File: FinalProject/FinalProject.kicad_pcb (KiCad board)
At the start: 4 copper layers, 100 x 100 mm, 143 parts, among them J1 GSB4111312HR, J10 Conn_01x02, J2 GSB4111312HR, J3 GSB4111312HR, J5 ARJM11D7-502-AB-EW2, J6 DCJ200-10-A-XX-K_REVA, J7 Conn_01x02, J9 Conn_01x03, Q1 NTTFS5C673NLTAG, Q2 NTTFS5C673NLTAG, SW2 SW_Push, U1 RTL8153B-VB-CG, U11 RP2040, U12 TUSB8041, U14 NCP1117-3.3_SOT223, U15 VEML6040, U16 MAX98357A, U2 TPS2561DRCR, U3 LM74700, U4 TPS62902RPJR, U5 LM74700, U8 ABM8-272-T3, U9 W25Q128JVS, Y2 ABLS-25.000MHZ-B2F-T, Y3 ABM3C-24.000MHZ-D4Y-T

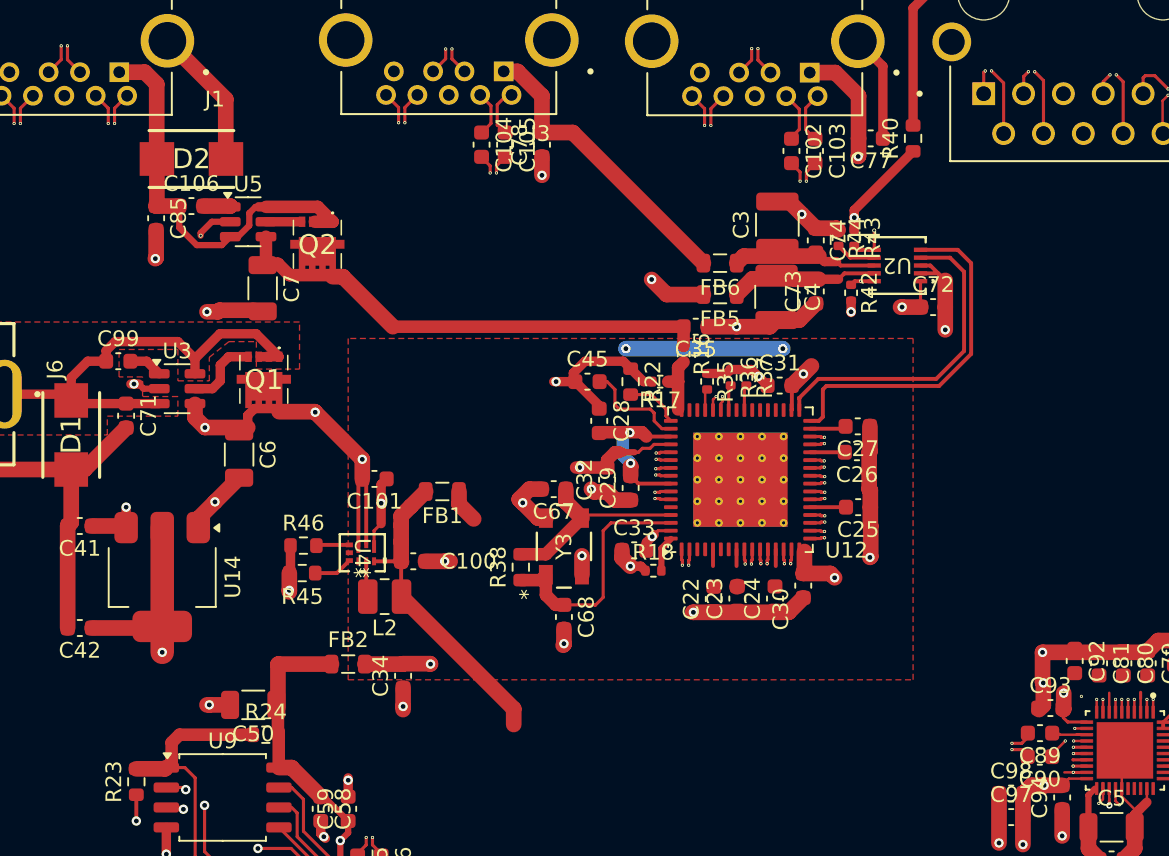
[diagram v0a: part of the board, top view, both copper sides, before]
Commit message: having DRC error
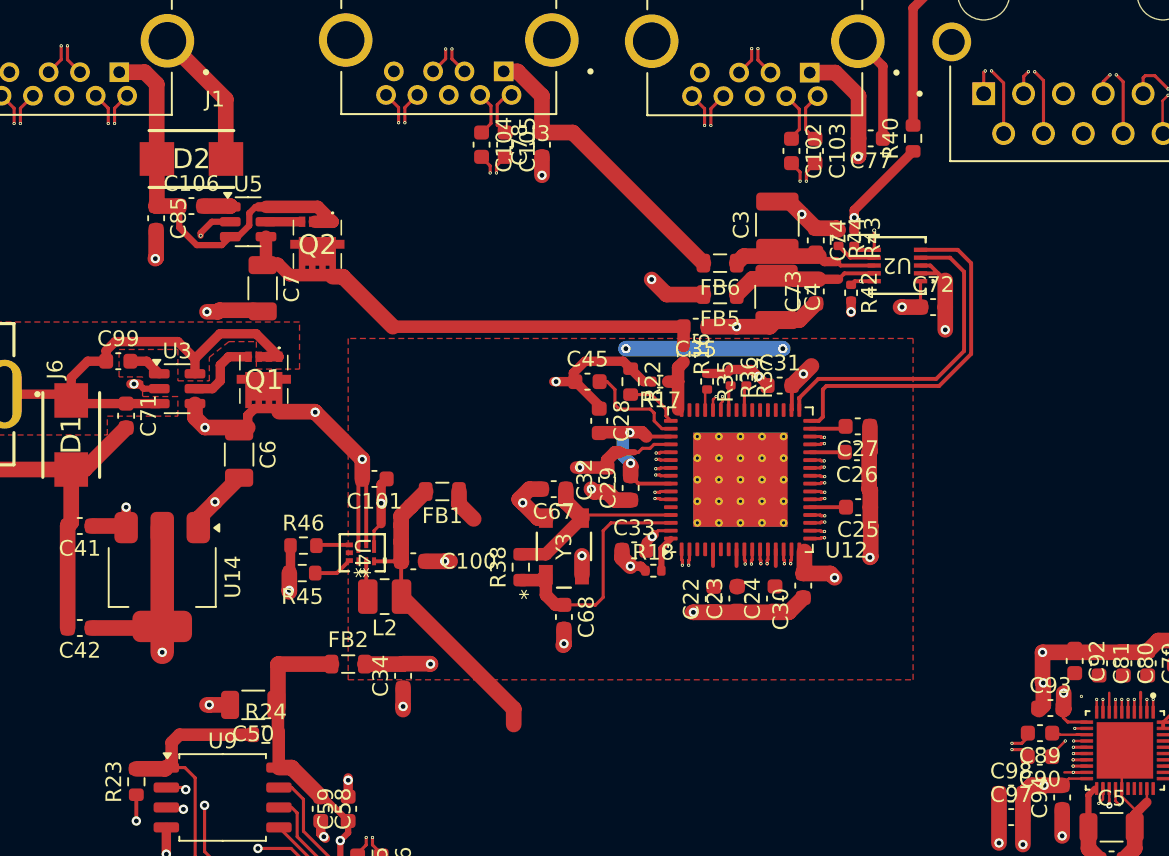
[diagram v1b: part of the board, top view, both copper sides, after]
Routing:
- net /DN1_D-: vias 1 -> 2
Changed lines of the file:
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@@
+	)
+	(via
+		(at 106.7 107.6)
+		(size 0.2)
+		(drill 0.1)
+		(layers "F.Cu" "B.Cu")
+		(net 101)
 	)
 	(via
@@
 	)
 	(segment
+		(start 81.0625 91)
+		(end 80.406249 91)
+		(width 0.2)
+		(layer "F.Cu")
+		(net 141)
+	)
+	(segment
 		(start 39.2125 67.05)
 		(end 39.2125 66.08)
@@
 		(start 39.2125 66.08)
 		(end 38.4125 65.28)
-		(width 0.2)
-		(layer "F.Cu")
-		(net 141)
-	)
-	(segment
-		(start 81.0625 91)
-		(end 80.406249 91)
 		(width 0.2)
 		(layer "F.Cu")
@@
 	)
 	(segment
+		(start 39.2125 68.245344)
+		(end 40.317156 69.35)
+		(width 0.2)
+		(layer "In2.Cu")
+		(net 141)
+	)
+	(segment
+		(start 68.517156 94)
+		(end 74.082844 94)
+		(width 0.2)
+		(layer "In2.Cu")
+		(net 141)
+	)
+	(segment
+		(start 77.132844 90.95)
+		(end 80.05 90.95)
+		(width 0.2)
+		(layer "In2.Cu")
+		(net 141)
+	)
+	(segment
+		(start 74.082844 94)
+		(end 77.132844 90.95)
+		(width 0.2)
+		(layer "In2.Cu")
+		(net 141)
+	)
+	(segment
+		(start 39.2125 67.05)
+		(end 39.2125 68.245344)
+		(width 0.2)
+		(layer "In2.Cu")
+		(net 141)
+	)
+	(segment
+		(start 43.867156 69.35)
+		(end 68.517156 94)
+		(width 0.2)
+		(layer "In2.Cu")
+		(net 141)
+	)
+	(segment
 		(start 40.317156 69.35)
-		(end 39.2125 68.245344)
-		(width 0.2)
-		(layer "In2.Cu")
-		(net 141)
-	)
-	(segment
-		(start 68.517156 94)
 		(end 43.867156 69.35)
-		(width 0.2)
-		(layer "In2.Cu")
-		(net 141)
-	)
-	(segment
-		(start 77.132844 90.95)
-		(end 74.082844 94)
-		(width 0.2)
-		(layer "In2.Cu")
-		(net 141)
-	)
-	(segment
-		(start 80.05 90.95)
-		(end 77.132844 90.95)
-		(width 0.2)
-		(layer "In2.Cu")
-		(net 141)
-	)
-	(segment
-		(start 74.082844 94)
-		(end 68.517156 94)
-		(width 0.2)
-		(layer "In2.Cu")
-		(net 141)
-	)
-	(segment
-		(start 39.2125 68.245344)
-		(end 39.2125 67.05)
-		(width 0.2)
-		(layer "In2.Cu")
-		(net 141)
-	)
-	(segment
-		(start 43.867156 69.35)
-		(end 40.317156 69.35)
 		(width 0.2)
 		(layer "In2.Cu")
@@
 	)
 	(segment
+		(start 45.2125 66.08)
+		(end 45.2125 67.05)
+		(width 0.2)
+		(layer "F.Cu")
+		(net 144)
+	)
+	(segment
 		(start 80.406249 89.5)
 		(end 80.356249 89.45)
@@
 	)
 	(segment
-		(start 45.2125 67.05)
+		(start 44.4125 65.28)
 		(end 45.2125 66.08)
-		(width 0.2)
-		(layer "F.Cu")
-		(net 144)
-	)
-	(segment
-		(start 45.2125 66.08)
-		(end 44.4125 65.28)
 		(width 0.2)
 		(layer "F.Cu")
@@
 	)
 	(segment
+		(start 79.182844 89.45)
+		(end 80.1 89.45)
+		(width 0.2)
+		(layer "In2.Cu")
+		(net 144)
+	)
+	(segment
+		(start 78.75413 89.878714)
+		(end 79.182844 89.45)
+		(width 0.2)
+		(layer "In2.Cu")
+		(net 144)
+	)
+	(segment
+		(start 77.49587 89.878714)
+		(end 78.75413 89.878714)
+		(width 0.2)
+		(layer "In2.Cu")
+		(net 144)
+	)
+	(segment
+		(start 73.667156 86.05)
+		(end 77.49587 89.878714)
+		(width 0.2)
+		(layer "In2.Cu")
+		(net 144)
+	)
+	(segment
 		(start 45.2125 67.545344)
 		(end 63.717156 86.05)
@@
 	)
 	(segment
-		(start 73.667156 86.05)
-		(end 77.49587 89.878714)
-		(width 0.2)
-		(layer "In2.Cu")
-		(net 144)
-	)
-	(segment
-		(start 78.75413 89.878714)
-		(end 79.182844 89.45)
-		(width 0.2)
-		(layer "In2.Cu")
-		(net 144)
-	)
-	(segment
-		(start 77.49587 89.878714)
-		(end 78.75413 89.878714)
-		(width 0.2)
-		(layer "In2.Cu")
-		(net 144)
-	)
-	(segment
-		(start 79.182844 89.45)
-		(end 80.1 89.45)
+		(start 45.2125 67.05)
+		(end 45.2125 67.545344)
 		(width 0.2)
 		(layer "In2.Cu")
@@
 		(width 0.2)
 		(layer "In2.Cu")
-		(net 144)
-	)
-	(segment
-		(start 45.2125 67.05)
-		(end 45.2125 67.545344)
-		(width 0.2)
-		(layer "In2.Cu")
